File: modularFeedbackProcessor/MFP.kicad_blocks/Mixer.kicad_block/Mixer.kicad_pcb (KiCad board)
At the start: 4 copper layers, 50 parts, among them Q11 Q_NMOS_GDS, Q12 Q_PMOS_GDS, Q13 Q_PMOS_GDS, Q14 Q_NMOS_GDS, Q15 Q_PMOS_GDS, Q16 Q_NMOS_GDS, Q17 Q_PMOS_GDS, Q18 Q_NMOS_GDS, Q19 Q_PMOS_GDS, U10 LM13700, U9 TL074

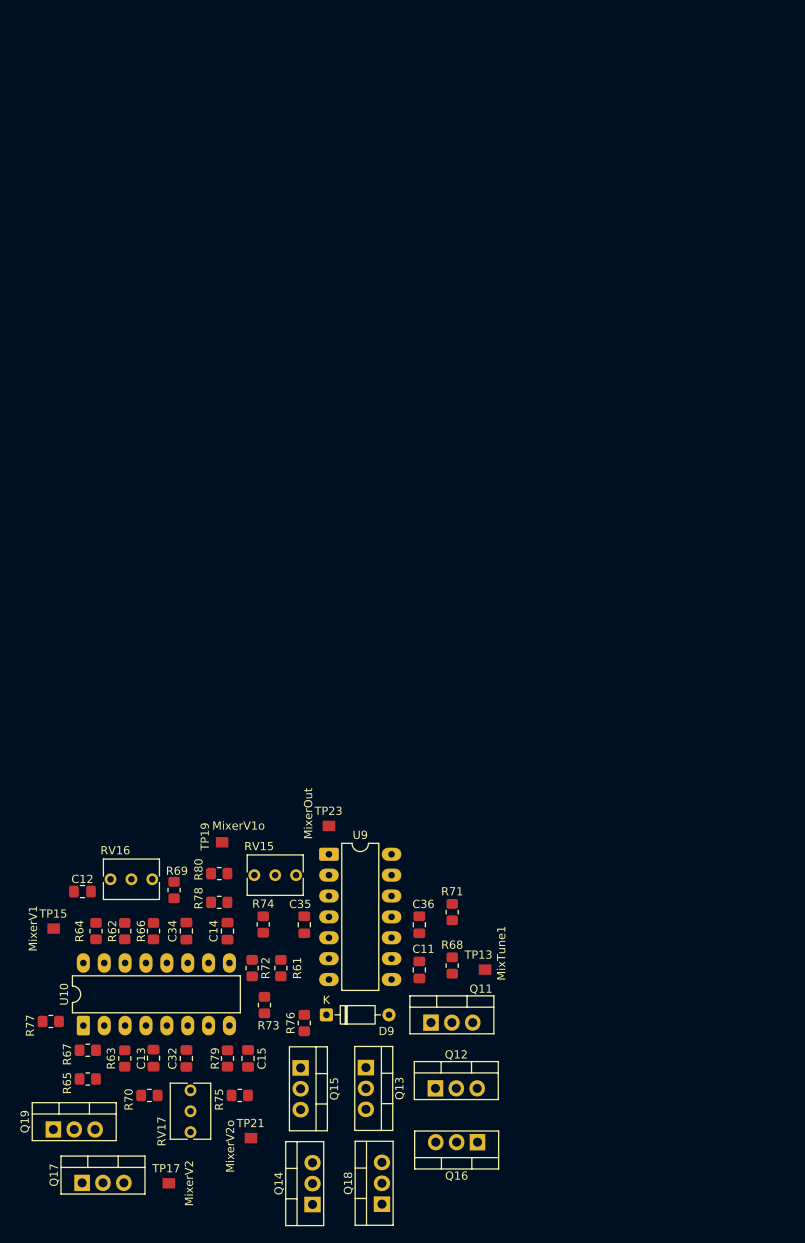
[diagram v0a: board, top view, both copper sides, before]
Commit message: Update: did not destroy everything
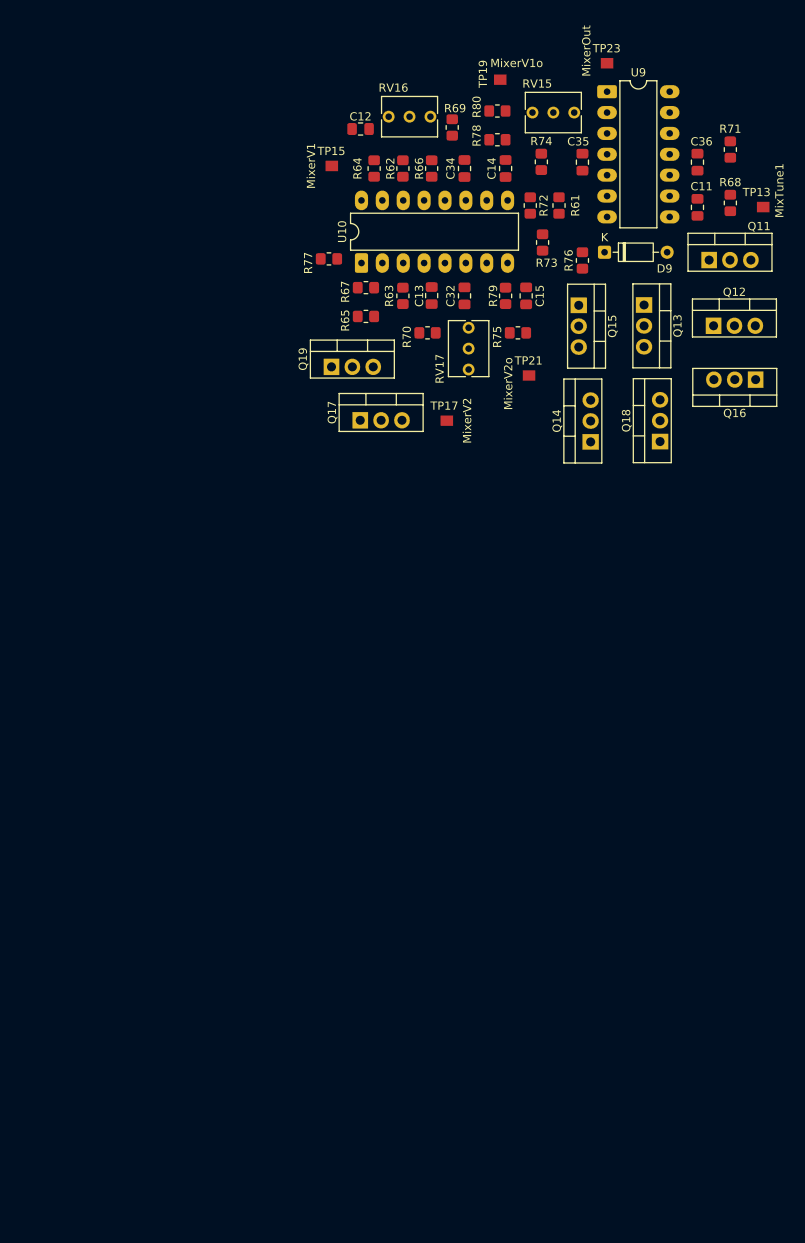
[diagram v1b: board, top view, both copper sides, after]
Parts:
- moved C11 98.8 mm to (357.4, -123.3)
- moved C12 98.8 mm to (316.4, -132.8)
- moved C13 98.8 mm to (325.0, -112.5)
- moved C14 98.8 mm to (334.0, -128.0)
- moved C15 98.8 mm to (336.5, -112.5)
- moved C32 98.8 mm to (329.0, -112.5)
- moved C34 98.8 mm to (329.0, -128.0)
- moved C35 98.8 mm to (343.4, -128.8)
- moved C36 98.8 mm to (357.4, -128.8)
- moved D9 98.8 mm to (346.0, -117.8)
- moved Q12 98.8 mm to (359.3, -108.9)
- moved Q13 98.8 mm to (350.9, -111.4)
- moved Q14 98.8 mm to (344.4, -94.7)
- moved Q16 98.8 mm to (364.4, -102.3)
- moved Q17 98.8 mm to (316.3, -97.4)
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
